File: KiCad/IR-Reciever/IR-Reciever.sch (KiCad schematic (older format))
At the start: 6 parts, among them P1 CONN_6, U1 TSOP38238, U2 TSOP38238, U3 TSOP38238, U4 RGBLED

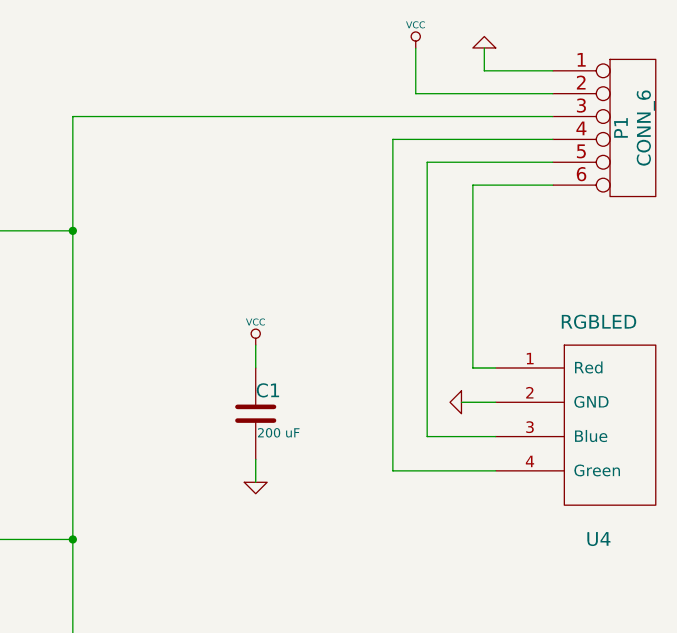
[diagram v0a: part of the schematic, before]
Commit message: Quick Update #2 5/1
Night night
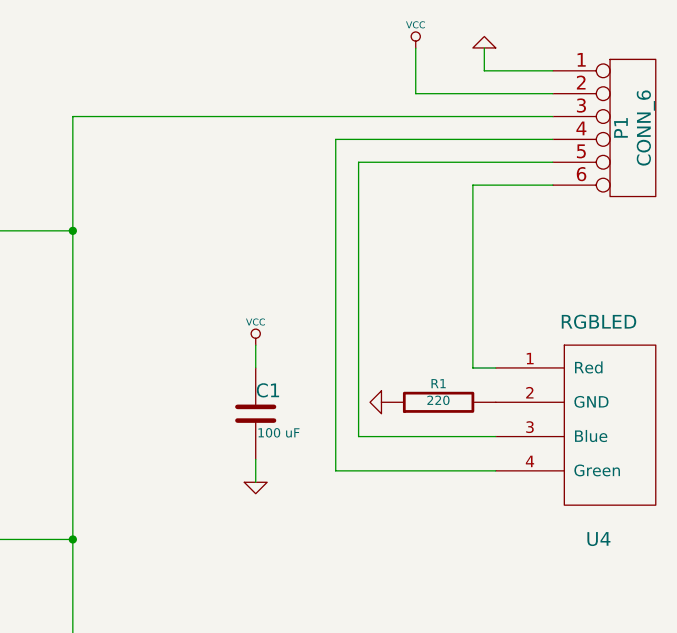
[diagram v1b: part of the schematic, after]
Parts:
- added R1: 220, ~, symbol R
- C1: value 200 uF -> 100 uF
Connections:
- net GND: now also R1.1; no longer U4.2 (GND)
- new net: R1.2, U4.2 (GND)
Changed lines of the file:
@@
 Sheet 1 1
 Title ""
-Date "6 mar 2015"
+Date "1 may 2015"
 Rev ""
 Comp ""
@@
 L GND #PWR09
 U 1 1 54F95FA4
-P 5150 2400
-F 0 "#PWR09" H 5150 2400 30  0001 C CNN
-F 1 "GND" H 5150 2330 30  0001 C CNN
-F 2 "" H 5150 2400 60  0000 C CNN
-F 3 "" H 5150 2400 60  0000 C CNN
-	1    5150 2400
+P 4800 2400
+F 0 "#PWR09" H 4800 2400 30  0001 C CNN
+F 1 "GND" H 4800 2330 30  0001 C CNN
+F 2 "" H 4800 2400 60  0000 C CNN
+F 3 "" H 4800 2400 60  0000 C CNN
+	1    4800 2400
 	0    1    1    0
 $EndComp
@@
 Connection ~ 3450 1650
 Wire Wire Line
-	5150 2400 5300 2400
-Wire Wire Line
 	5550 1450 5200 1450
 Wire Wire Line
@@
 	5200 2250 5300 2250
 Wire Wire Line
-	5550 1350 5000 1350
-Wire Wire Line
-	5000 1350 5000 2550
-Wire Wire Line
-	5000 2550 5300 2550
-Wire Wire Line
-	5550 1250 4850 1250
-Wire Wire Line
-	4850 1250 4850 2700
-Wire Wire Line
-	4850 2700 5300 2700
+	4700 1350 5550 1350
+Wire Wire Line
+	4700 2550 5300 2550
+Wire Wire Line
+	4600 1250 5550 1250
+Wire Wire Line
+	4600 2700 5300 2700
 $Comp
 L VCC #PWR010
@@
 P 4250 2450
 F 0 "C1" H 4250 2550 60  0000 L CNN
-F 1 "200 uF" H 4256 2365 40  0000 L CNN
+F 1 "100 uF" H 4256 2365 40  0000 L CNN
 F 2 "~" H 4288 2300 30  0000 C CNN
 F 3 "~" H 4250 2450 60  0000 C CNN
@@
 Wire Wire Line
 	4250 2650 4250 2750
+$Comp
+L R R1
+U 1 1 554311D1
+P 5050 2400
+F 0 "R1" V 5130 2400 40  0000 C CNN
+F 1 "220" V 5057 2401 40  0000 C CNN
+F 2 "~" V 4980 2400 30  0000 C CNN
+F 3 "~" H 5050 2400 30  0000 C CNN
+	1    5050 2400
+	0    -1   -1   0
+$EndComp
+Wire Wire Line
+	4700 2550 4700 1350
+Wire Wire Line
+	4600 1250 4600 2700
 $EndSCHEMATC
